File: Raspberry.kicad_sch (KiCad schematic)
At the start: 31 parts, among them J11 CAN, J18 SPARE_RASPI, J19 Raspberry_Pi_2_3, J20 RASPI_FAN, Q16 2N7002NXAK, Q2 2N7002NXAK, U3 PCA9634PW,118, U4 MCP2515-xSO, U5 MCP2562-E-SN, Y1 16MHz

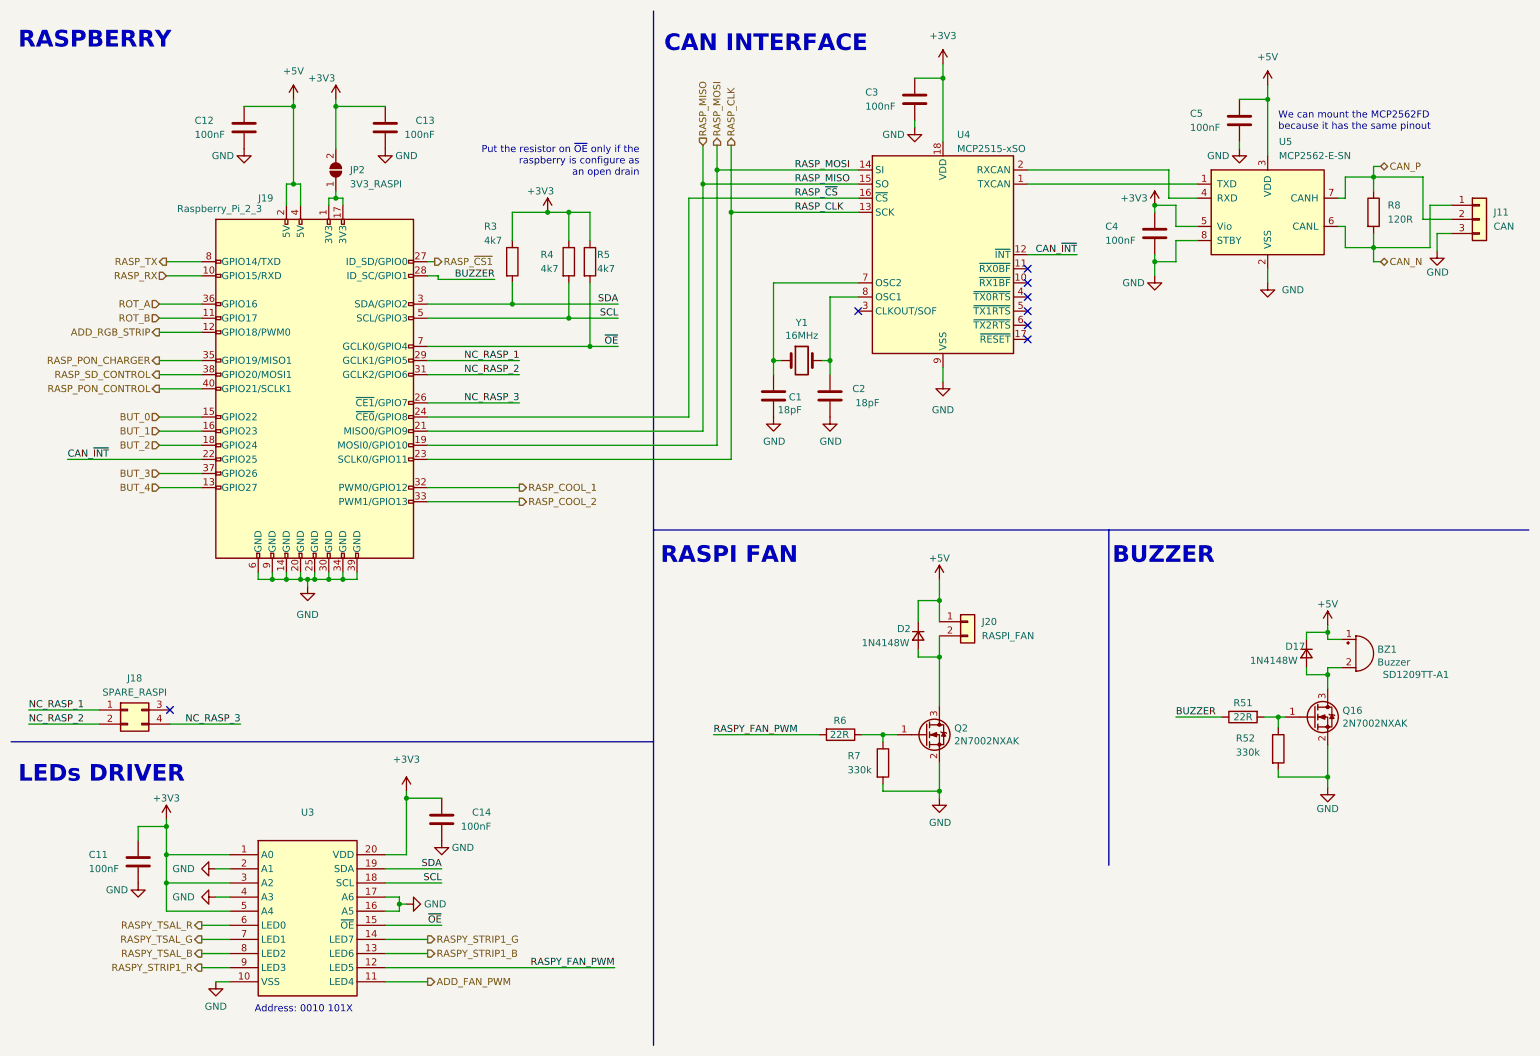
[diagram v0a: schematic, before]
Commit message: Fixed Schematic, fixed some traces. Still not finished
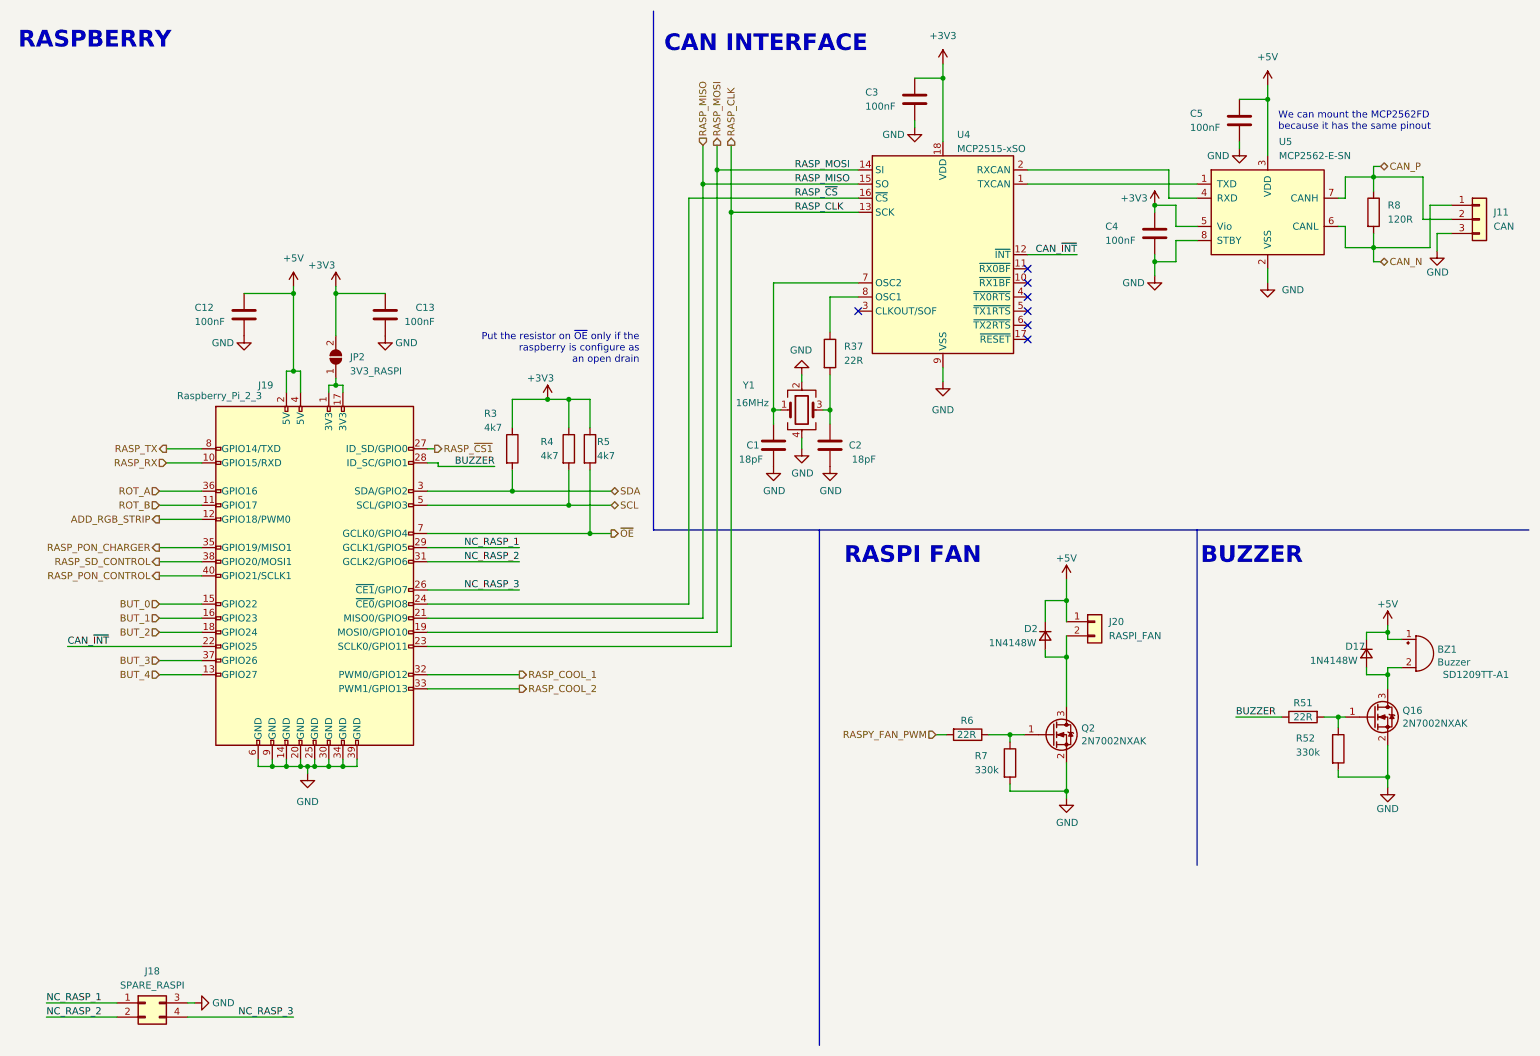
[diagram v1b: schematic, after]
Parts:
- removed C11, C14: 100nF, Resistor_SMD:R_0805_2012Metric, symbol Device:C
- removed U3: PCA9634PW,118, 00_proj-lib:SOP65P640X110-20N, symbol 00_proj-lib:PCA9634PW,118
- added R37: 22R, Resistor_SMD:R_0603_1608Metric, symbol Device:R
- C1, C2: footprint Resistor_SMD:R_0603_1608Metric -> Capacitor_SMD:C_0603_1608Metric
- C12, C13, C3, C4, C5: footprint Resistor_SMD:R_0805_2012Metric -> Capacitor_SMD:C_0603_1608Metric
- D17, D2: footprint Diode_SMD:D_SOD-323_HandSoldering -> Diode_SMD:D_SOD-123
- Y1: footprint Crystal:Crystal_HC49-4H_Vertical -> Crystal:Crystal_SMD_3225-4Pin_3.2x2.5mm; symbol Device:Crystal -> Device:Crystal_GND24; Campo4 (none) -> ECS-160-18-33-AEN-TR
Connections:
- net GND: now also J18.3 (Pin_3), Y1.2, Y1.4
- new net: C2.1, R37.2, Y1.3
- new net: R37.1, U4.8 (OSC1)
- no-connect marks 8 -> 7
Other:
- note removed: "Address: 0010 101X"
- note removed: "LEDs DRIVER"
- moved on the sheet: BZ1, C1, C12, C13, C2, D17, D2, J18, J19, J20, JP2, Q16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
